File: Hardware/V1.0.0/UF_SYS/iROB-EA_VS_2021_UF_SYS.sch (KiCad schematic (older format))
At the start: 33 parts

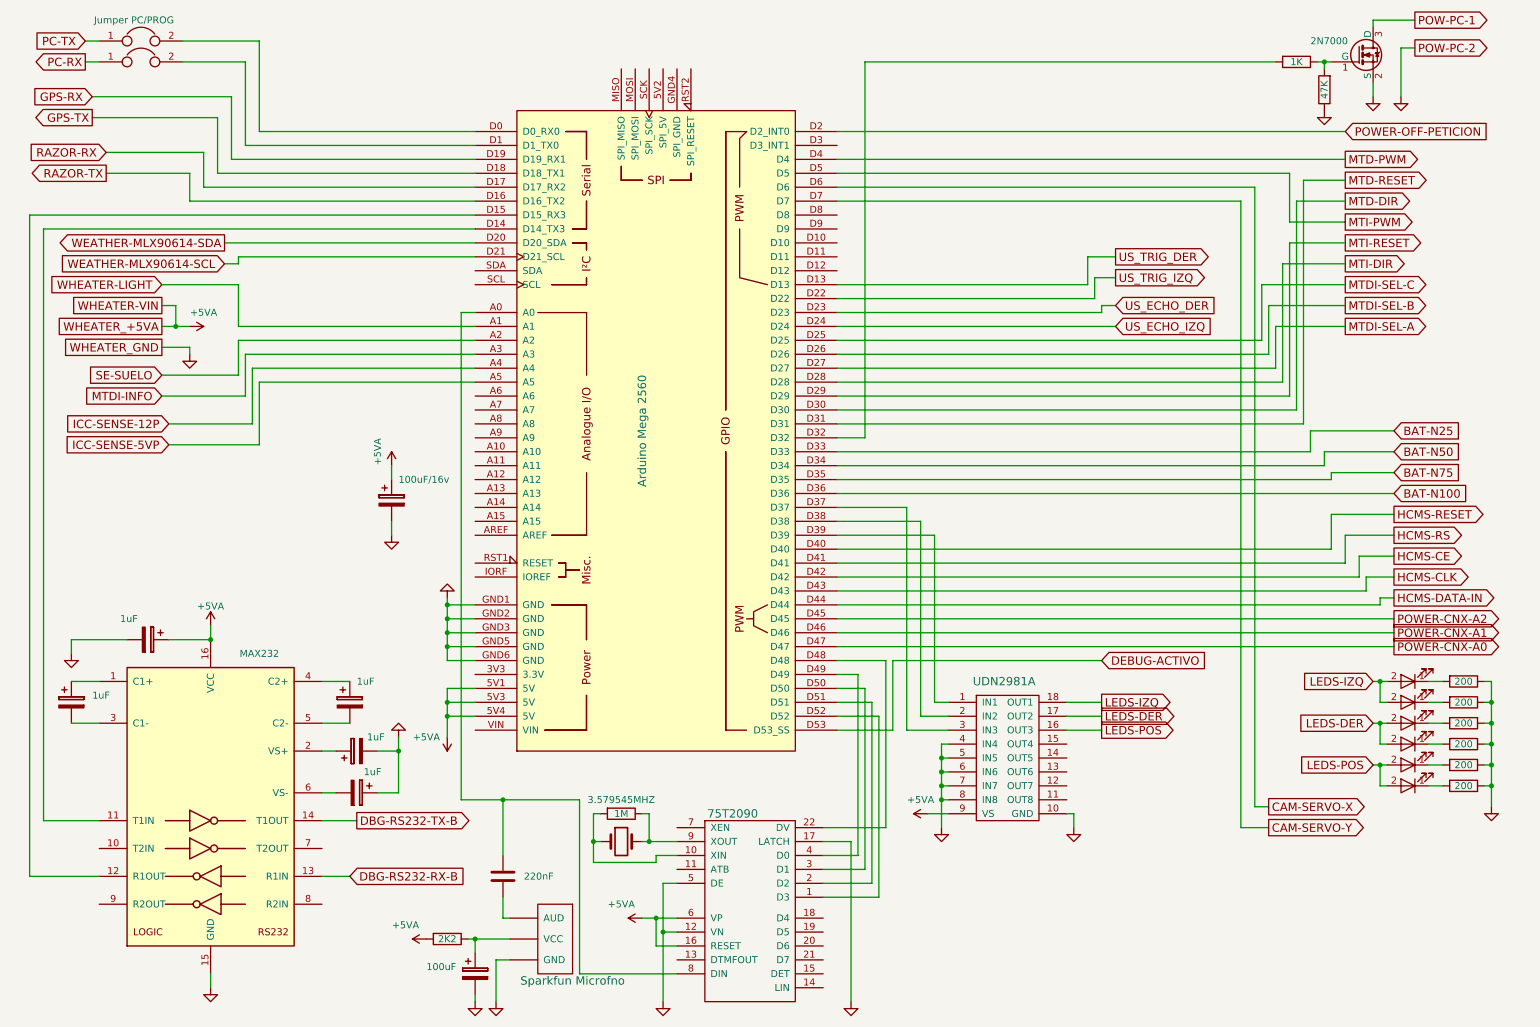
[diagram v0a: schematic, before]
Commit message: Actualizacion 2021
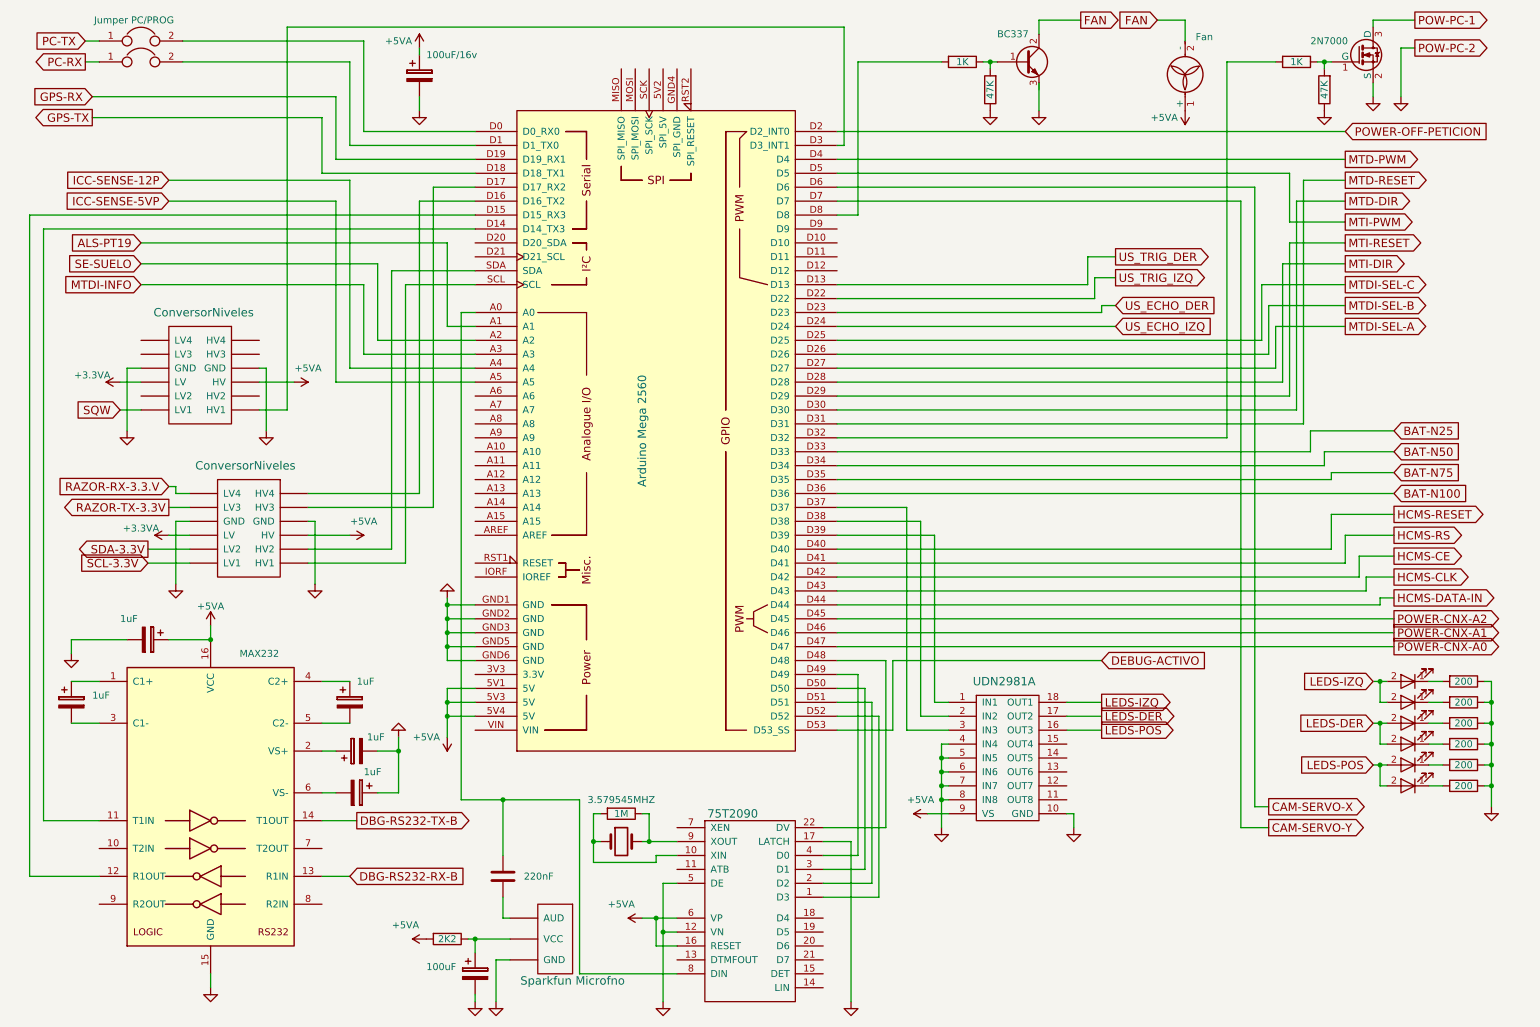
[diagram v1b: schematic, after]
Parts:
- added M?: Fan, symbol Fan
- added Q?: BC337, symbol Q_NPN_BCE
- added R?: 1K, symbol R
- added R?: 47K, symbol R
- added U? (x2): ConversorNiveles, symbol ConversorNiveles
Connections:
- net +5VA: now also M?.1 (+), U?.~ (LV4), U?.~ (LV4)
- net GND: now also R?.1, U?.~ (LV4), U?.~ (LV4)
- net at XA?.D3 (D3_INT1): now also U?.~ (LV4)
- net at XA?.D8: now also R?.2
- net at XA?.SCL: now also U?.~ (LV4)
- net at XA?.SDA: now also U?.~ (LV4)
- net RAZOR-RX: no longer names the net of XA?.D17 (D17_RX2)
- net RAZOR-RX: now also U?.~ (LV4)
- net RAZOR-TX: no longer names the net of XA?.D16 (D16_TX2)
- net RAZOR-TX: now also U?.~ (LV4)
- net WEATHER-MLX90614-SCL: no longer names the net of XA?.D21 (D21_SCL)
- net WEATHER-MLX90614-SDA: no longer names the net of XA?.D20 (D20_SDA)
- net WHEATER-LIGHT renamed ALS-PT19
- new net: Q?.1 (B), R?.1, R?.2
- new net +3.3VA: U?.~ (LV4), U?.~ (LV4)
- new net FAN: M?.2 (-), Q?.2 (C)
- new net RAZOR-RX-3.3.V: U?.~ (LV4)
- new net RAZOR-TX-3.3V: U?.~ (LV4)
- new net SCL-3.3V: U?.~ (LV4)
- new net SDA-3.3V: U?.~ (LV4)
- new net SQW: U?.~ (LV4)

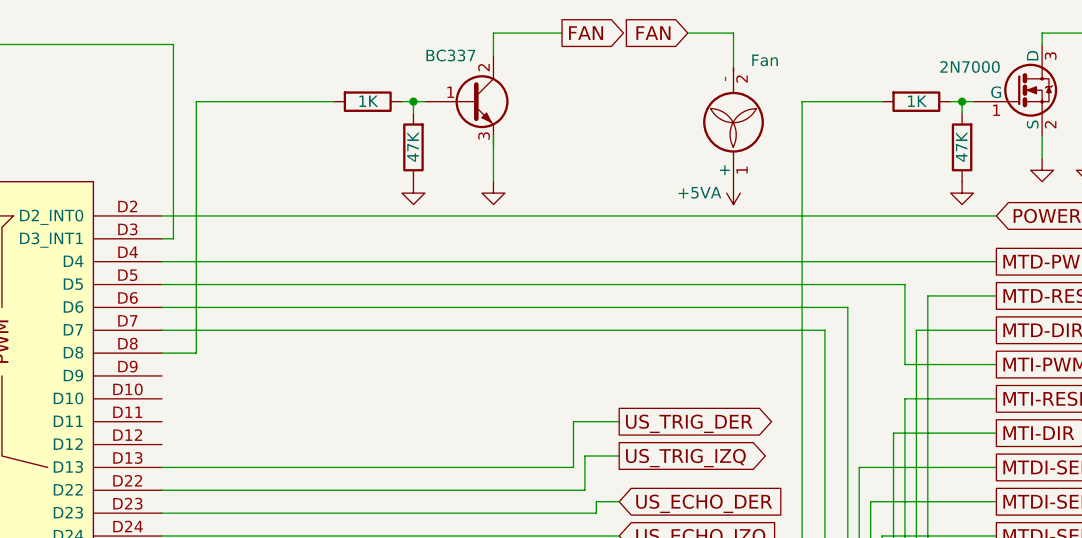
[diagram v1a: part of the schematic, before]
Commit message: Actualizacion ficheros CAD
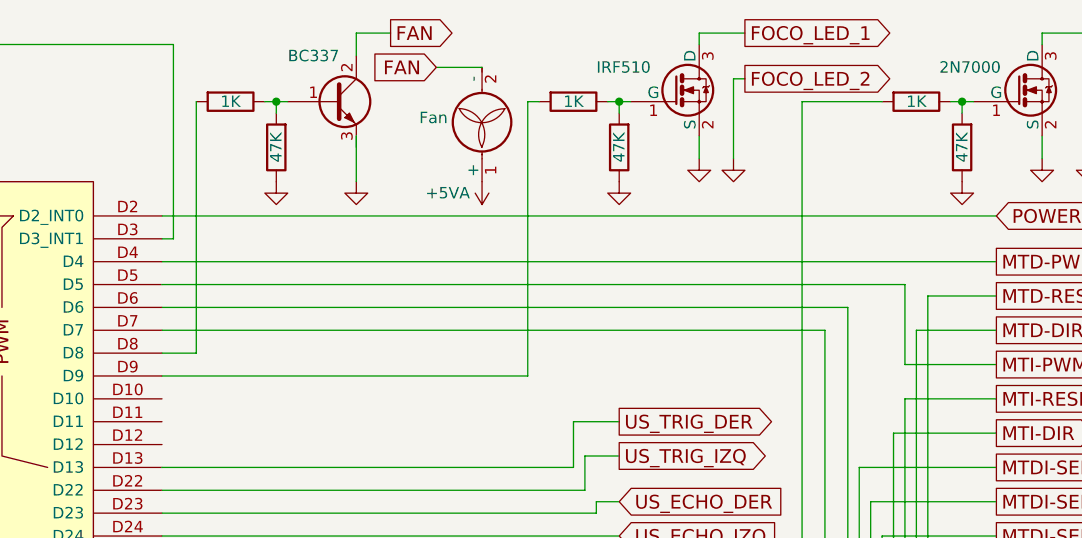
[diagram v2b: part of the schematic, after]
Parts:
- added Q?: IRF510, TO_SOT_Packages_SMD:SOT-23, symbol 2N7002
- added R?: 1K, symbol R
- added R?: 47K, symbol R
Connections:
- net GND: now also Q?.2 (S), R?.1
- net at XA?.D9: now also R?.2
- new net: Q?.1 (G), R?.1, R?.2
- new net FOCO_LED_1: Q?.3 (D)
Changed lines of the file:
@@
 L GND #PWR?
 U 1 1 608FBD35
-P 7850 1200
-F 0 "#PWR?" H 7850 950 50  0001 C CNN
-F 1 "GND" H 7850 1050 50  0001 C CNN
-F 2 "" H 7850 1200 50  0000 C CNN
-F 3 "" H 7850 1200 50  0000 C CNN
-	1    7850 1200
+P 7250 1200
+F 0 "#PWR?" H 7250 950 50  0001 C CNN
+F 1 "GND" H 7250 1050 50  0001 C CNN
+F 2 "" H 7250 1200 50  0000 C CNN
+F 3 "" H 7250 1200 50  0000 C CNN
+	1    7250 1200
 	1    0    0    -1
 $EndComp
@@
 L R R?
 U 1 1 608FBD3B
-P 7300 850
-F 0 "R?" V 7380 850 50  0001 C CNN
-F 1 "1K" V 7300 850 50  0000 C CNN
-F 2 "" V 7230 850 50  0000 C CNN
-F 3 "" H 7300 850 50  0000 C CNN
-	1    7300 850
+P 6700 850
+F 0 "R?" V 6780 850 50  0001 C CNN
+F 1 "1K" V 6700 850 50  0000 C CNN
+F 2 "" V 6630 850 50  0000 C CNN
+F 3 "" H 6700 850 50  0000 C CNN
+	1    6700 850
 	0    1    1    0
 $EndComp
 Wire Wire Line
-	7450 850  7550 850
-Wire Wire Line
-	8150 550  7850 550
-Wire Wire Line
-	7850 550  7850 650
+	6850 850  6950 850
+Wire Wire Line
+	7250 550  7250 650
 $Comp
 L R R?
 U 1 1 608FBD44
-P 7500 1050
-F 0 "R?" V 7580 1050 50  0001 C CNN
-F 1 "47K" V 7500 1050 50  0000 C CNN
-F 2 "" V 7430 1050 50  0000 C CNN
-F 3 "" H 7500 1050 50  0000 C CNN
-	1    7500 1050
+P 6900 1050
+F 0 "R?" V 6980 1050 50  0001 C CNN
+F 1 "47K" V 6900 1050 50  0000 C CNN
+F 2 "" V 6830 1050 50  0000 C CNN
+F 3 "" H 6900 1050 50  0000 C CNN
+	1    6900 1050
 	-1   0    0    1
 $EndComp
 Wire Wire Line
-	7500 900  7500 850
-Connection ~ 7500 850
+	6900 900  6900 850
+Connection ~ 6900 850
 $Comp
 L GND #PWR?
 U 1 1 608FBD4C
-P 7500 1200
-F 0 "#PWR?" H 7500 950 50  0001 C CNN
-F 1 "GND" H 7500 1050 50  0001 C CNN
-F 2 "" H 7500 1200 50  0000 C CNN
-F 3 "" H 7500 1200 50  0000 C CNN
-	1    7500 1200
-	1    0    0    -1
-$EndComp
-Wire Wire Line
-	7850 1000 7850 1200
-Text GLabel 8150 550  2    60   Output ~ 0
+P 6900 1200
+F 0 "#PWR?" H 6900 950 50  0001 C CNN
+F 1 "GND" H 6900 1050 50  0001 C CNN
+F 2 "" H 6900 1200 50  0000 C CNN
+F 3 "" H 6900 1200 50  0000 C CNN
+	1    6900 1200
+	1    0    0    -1
+$EndComp
+Wire Wire Line
+	7250 1000 7250 1200
+Text GLabel 7400 550  2    60   Output ~ 0
 FAN
 Wire Wire Line
@@
 L Fan M?
 U 1 1 6092DF2C
-P 8900 900
-F 0 "M?" H 9000 1100 50  0001 L CNN
-F 1 "Fan" H 8700 700 50  0000 L TNN
-F 2 "" H 8900 910 50  0001 C CNN
-F 3 "" H 8900 910 50  0001 C CNN
-	1    8900 900
+P 7800 900
+F 0 "M?" H 7900 1100 50  0001 L CNN
+F 1 "Fan" H 7950 950 50  0000 L TNN
+F 2 "" H 7800 910 50  0001 C CNN
+F 3 "" H 7800 910 50  0001 C CNN
+	1    7800 900
 	-1   0    0    1
 $EndComp
-Wire Wire Line
-	7150 850  6550 850
 $Comp
 L Q_NPN_BCE Q?
 U 1 1 6092E108
-P 7750 850
-F 0 "Q?" H 7550 950 50  0001 L CNN
-F 1 "BC337" H 7550 1050 50  0000 L CNN
-F 2 "" H 7950 950 50  0000 C CNN
-F 3 "" H 7750 850 50  0000 C CNN
-	1    7750 850
-	1    0    0    -1
-$EndComp
-Text GLabel 8700 550  0    60   Input ~ 0
+P 7150 850
+F 0 "Q?" H 6950 950 50  0001 L CNN
+F 1 "BC337" H 6950 1050 50  0000 L CNN
+F 2 "" H 7350 950 50  0000 C CNN
+F 3 "" H 7150 850 50  0000 C CNN
+	1    7150 850
+	1    0    0    -1
+$EndComp
+Text GLabel 7600 700  0    60   Input ~ 0
 FAN
-Wire Wire Line
-	8700 550  8900 550
-Wire Wire Line
-	8900 550  8900 700
 $Comp
 L +5VA #PWR?
 U 1 1 6092E465
-P 8900 1200
-F 0 "#PWR?" H 8900 1050 50  0001 C CNN
-F 1 "+5VA" H 9050 1250 50  0000 C CNN
-F 2 "" H 8900 1200 50  0000 C CNN
-F 3 "" H 8900 1200 50  0000 C CNN
-	1    8900 1200
+P 7800 1200
+F 0 "#PWR?" H 7800 1050 50  0001 C CNN
+F 1 "+5VA" H 7950 1250 50  0000 C CNN
+F 2 "" H 7800 1200 50  0000 C CNN
+F 3 "" H 7800 1200 50  0000 C CNN
+	1    7800 1200
 	-1   0    0    1
 $EndComp
@@
 Wire Wire Line
 	1250 3350 1400 3350
+Wire Wire Line
+	7600 700  7800 700
+Wire Wire Line
+	7250 550  7400 550
+$Comp
+L 2N7002 Q?
+U 1 1 618A5AC0
+P 8650 800
+F 0 "Q?" H 8850 875 50  0001 L CNN
+F 1 "IRF510" H 8300 900 50  0000 L CNN
+F 2 "TO_SOT_Packages_SMD:SOT-23" H 8850 725 50  0001 L CIN
+F 3 "" H 8650 800 50  0000 L CNN
+	1    8650 800
+	1    0    0    -1
+$EndComp
+$Comp
+L GND #PWR?
+U 1 1 618A5AC6
+P 8750 1100
+F 0 "#PWR?" H 8750 850 50  0001 C CNN
+F 1 "GND" H 8750 950 50  0001 C CNN
+F 2 "" H 8750 1100 50  0000 C CNN
+F 3 "" H 8750 1100 50  0000 C CNN
+	1    8750 1100
+	1    0    0    -1
+$EndComp
+$Comp
+L R R?
+U 1 1 618A5ACC
+P 8200 850
+F 0 "R?" V 8280 850 50  0001 C CNN
+F 1 "1K" V 8200 850 50  0000 C CNN
+F 2 "" V 8130 850 50  0000 C CNN
+F 3 "" H 8200 850 50  0000 C CNN
+	1    8200 850
+	0    1    1    0
+$EndComp
+Wire Wire Line
+	8350 850  8450 850
+Wire Wire Line
+	8750 550  8750 600
+$Comp
+L GND #PWR?
+U 1 1 618A5AD4
+P 8900 1100
+F 0 "#PWR?" H 8900 850 50  0001 C CNN
+F 1 "GND" H 8900 950 50  0001 C CNN
+F 2 "" H 8900 1100 50  0000 C CNN
+F 3 "" H 8900 1100 50  0000 C CNN
+	1    8900 1100
+	1    0    0    -1
+$EndComp
+$Comp
+L R R?
+U 1 1 618A5ADB
+P 8400 1050
+F 0 "R?" V 8480 1050 50  0001 C CNN
+F 1 "47K" V 8400 1050 50  0000 C CNN
+F 2 "" V 8330 1050 50  0000 C CNN
+F 3 "" H 8400 1050 50  0000 C CNN
+	1    8400 1050
+	-1   0    0    1
+$EndComp
+Wire Wire Line
+	8400 900  8400 850
+Connection ~ 8400 850
+$Comp
+L GND #PWR?
+U 1 1 618A5AE3
+P 8400 1200
+F 0 "#PWR?" H 8400 950 50  0001 C CNN
+F 1 "GND" H 8400 1050 50  0001 C CNN
+F 2 "" H 8400 1200 50  0000 C CNN
+F 3 "" H 8400 1200 50  0000 C CNN
+	1    8400 1200
+	1    0    0    -1
+$EndComp
+Wire Wire Line
+	8900 750  8900 1100
+Wire Wire Line
+	8750 1000 8750 1100
+Text GLabel 8950 550  2    60   Output ~ 0
+FOCO_LED_1
+Wire Wire Line
+	8750 550  8950 550
+Text GLabel 8950 750  2    60   Output ~ 0
+FOCO_LED_2
+Wire Wire Line
+	8900 750  8950 750
+Wire Wire Line
+	8050 850  8000 850
+Wire Wire Line
+	8000 850  8000 2050
+Wire Wire Line
+	8000 2050 6400 2050
 $EndSCHEMATC

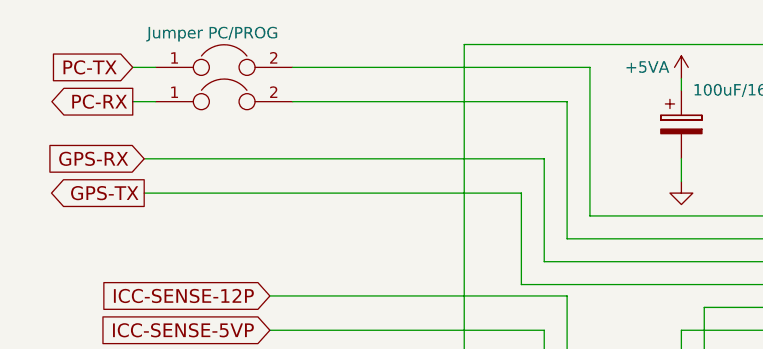
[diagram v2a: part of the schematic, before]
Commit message: Actualizacion python
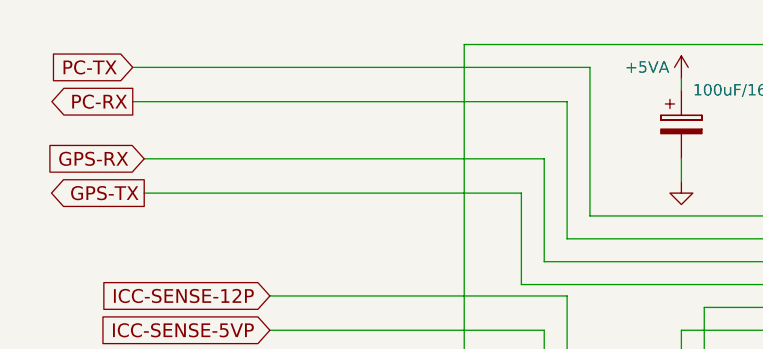
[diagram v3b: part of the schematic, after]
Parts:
- removed JP? (x2): Jumper PC/PROG, symbol Jumper
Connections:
- net PC-RX: now also XA?.D1 (D1_TX0)
- net PC-TX: now also XA?.D0 (D0_RX0)
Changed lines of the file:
@@
 	700  2050 700  6300
 Wire Wire Line
-	1000 700  1100 700
-Wire Wire Line
-	1700 700  3000 700
+	1000 700  3000 700
 Wire Wire Line
 	1050 1100 2800 1100
@@
 Text GLabel 1600 1850 0    60   Input ~ 0
 ICC-SENSE-5VP
-$Comp
-L Jumper JP?
-U 1 1 606DF3B4
-P 1400 850
-F 0 "JP?" H 1400 1000 50  0001 C CNN
-F 1 "Jumper PC/PROG" H 1350 1000 50  0001 C CNN
-F 2 "" H 1400 850 50  0000 C CNN
-F 3 "" H 1400 850 50  0000 C CNN
-	1    1400 850
-	1    0    0    -1
-$EndComp
-$Comp
-L Jumper JP?
-U 1 1 6064BD73
-P 1400 700
-F 0 "JP?" H 1400 850 50  0001 C CNN
-F 1 "Jumper PC/PROG" H 1350 850 50  0000 C CNN
-F 2 "" H 1400 700 50  0000 C CNN
-F 3 "" H 1400 700 50  0000 C CNN
-	1    1400 700
-	1    0    0    -1
-$EndComp
-Wire Wire Line
-	1100 850  1000 850
-Wire Wire Line
-	1700 850  2900 850
+Wire Wire Line
+	1000 850  2900 850
 Wire Wire Line
 	2700 6700 2900 6700
